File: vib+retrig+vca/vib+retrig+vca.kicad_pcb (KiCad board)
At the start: 2 copper layers, 49 parts, among them J1 Conn_01x10_MountingPin, J2 Conn_01x02_MountingPin, Q1 Q_NJFET_DSG, Q2 BC237, Q3 BC237, Q4 BC307, SW1 SW_SPDT, SW2 SW_SP3T, U1 TL072, U2 TL072, U3 CA3080

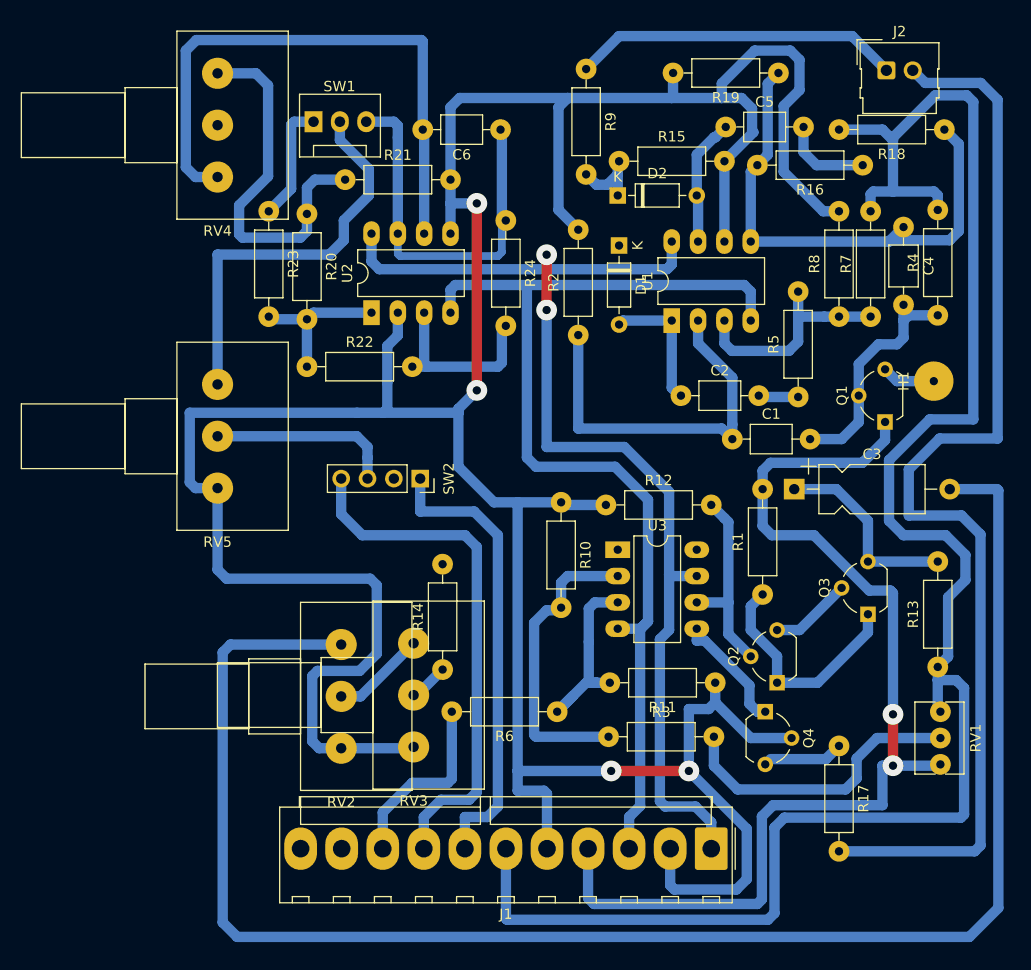
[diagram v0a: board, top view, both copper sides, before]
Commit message: Add files via upload
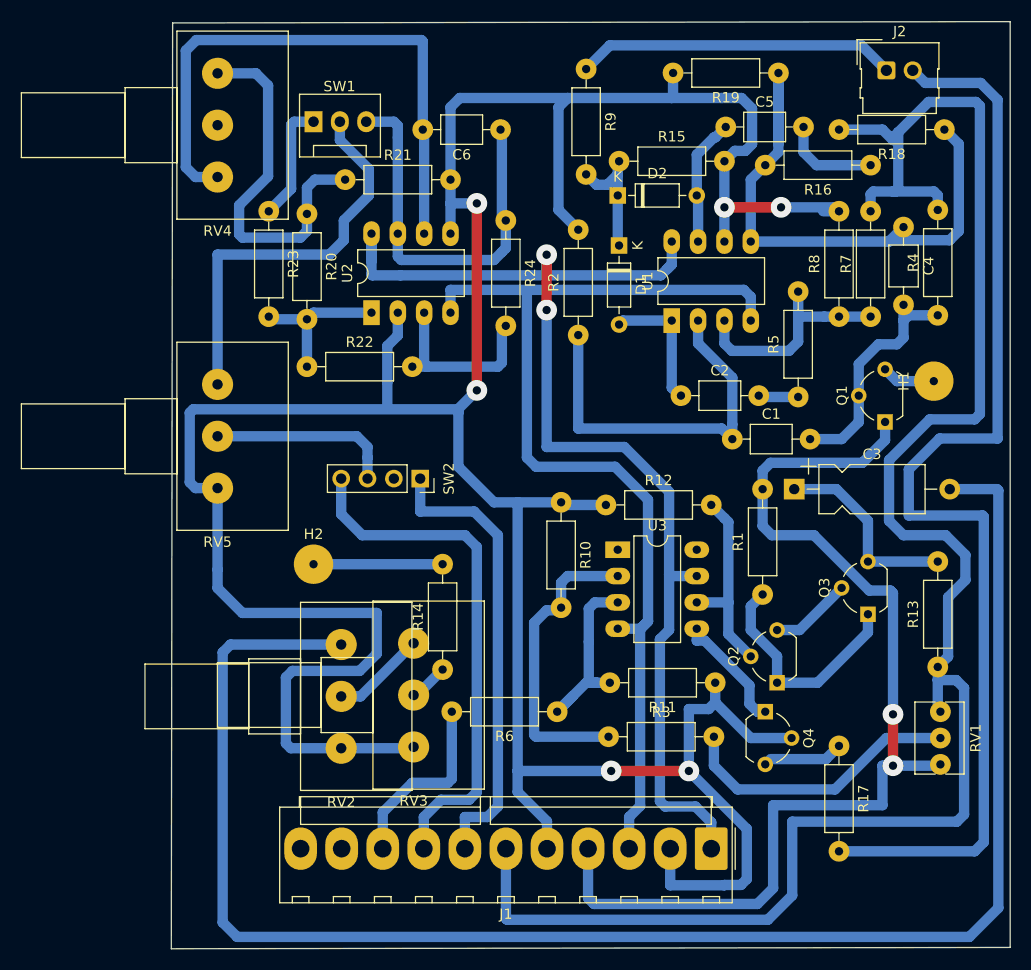
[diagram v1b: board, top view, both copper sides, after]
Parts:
- added H2: MountingHole_Pad, MountingHole:MountingHole_2.2mm_M2_DIN965_Pad, F.Cu at (77.6, 106.0)
- moved R16 0.76 mm to (131.3, 67.6)
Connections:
- R14 pad 2: (no net) -> Net-(H2-Pad1)
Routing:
- net GND: track 341.9 -> 328.6 mm, vias 4 -> 6
- net Net-(H2-Pad1): track 0.00 -> 12.4 mm
- net Net-(C4-Pad1): track 50.2 -> 57.0 mm
- net +15V: track 109.7 -> 116.3 mm
- net Net-(D1-Pad1): track 7.41 -> 12.3 mm
- net Net-(J2-Pad2): track 107.8 -> 109.3 mm
- net Net-(R3-Pad2): track 28.8 -> 27.6 mm
- net -15V: track 102.0 -> 101.0 mm
- net Net-(J2-Pad1): track 31.6 -> 30.9 mm
- net Net-(C6-Pad1): track 37.7 -> 38.3 mm
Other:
- board outline added: 80.9 x 89.4 mm
- net class Default: clearance 0.2 -> 0.4
- rule trace_clearance: 0.2 -> 0.4
